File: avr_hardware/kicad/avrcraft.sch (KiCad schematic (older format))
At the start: 55 parts, among them J1 AVRISP6, P1 ETHERNET, P2 CONN_1, P3 CONN_1, P4 CONN_1, P5 CONN_1, P6 CONN_1, P7 CONN_1, P8 CONN_1, Q1 MOSFET_P, T1 S553-5999-52, U1 ATMEGA328, U2 MCP1824, U3 ENC424J600, U4 A4447SLJTR, X1 XTAL4P, X2 25MHz

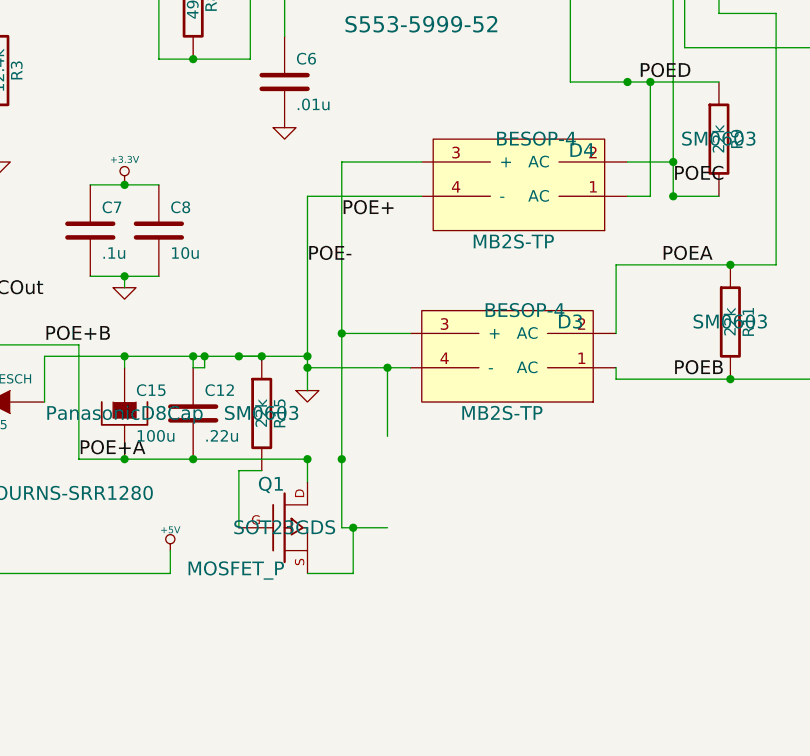
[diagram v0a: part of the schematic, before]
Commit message: update files for actual hardware
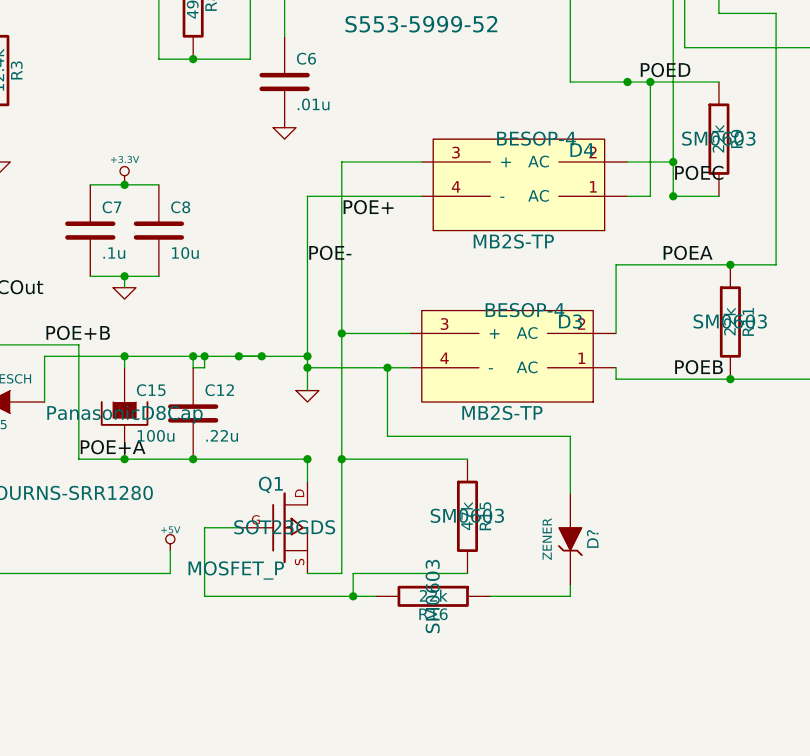
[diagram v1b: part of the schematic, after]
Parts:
- added D?: ZENER, symbol ZENER
- added R16: 22k, SM0603, symbol R
- C6: footprint SM0805 -> SM0603
- R15: value 22k -> 47k
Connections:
- net GND: now also D?.1 (A); no longer R15.1
- net POE+: now also R15.1
- net at Q1.G, R15.2: now also R16.2
- new net: D?.2 (K), R16.1
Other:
- moved on the sheet: R15
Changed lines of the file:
@@
-EESchema Schematic File Version 2  date Thu 31 Jan 2013 12:07:58 AM EST
+EESchema Schematic File Version 2  date Sun 03 Feb 2013 12:44:29 AM EST
 LIBS:power
 LIBS:device
@@
 LIBS:a4447sljtr
 LIBS:crystal-4p
+LIBS:zener-sot23-3
 LIBS:avrcraft-cache
 EELAYER 25  0
@@
 Sheet 1 1
 Title ""
-Date "31 jan 2013"
+Date "3 feb 2013"
 Rev ""
 Comp ""
@@
 Comment4 ""
 $EndDescr
-Text Label 7750 6450 0    60   ~ 0
-POE+A
+Wire Wire Line
+	9900 7000 9900 7050
+Wire Wire Line
+	8750 6950 8900 6950
+Wire Wire Line
+	8900 6950 8900 5150
+Wire Wire Line
+	9900 7050 9550 7050
 Wire Wire Line
 	8750 6450 7750 6450
@@
 Connection ~ 9100 6050
 Wire Wire Line
-	9100 6350 9100 6050
+	9100 6050 9100 6350
 Connection ~ 3800 1800
 Wire Wire Line
@@
 Connection ~ 10600 6100
 Wire Wire Line
-	9250 5150 8900 5150
+	8900 5150 9250 5150
 Wire Wire Line
 	9250 5300 8750 5300
@@
 Wire Wire Line
 	1400 2800 2000 2800
-Wire Wire Line
-	8900 5150 8900 6750
-Wire Wire Line
-	8900 6750 9100 6750
 Connection ~ 8900 6450
-Wire Wire Line
-	8750 6950 8950 6950
-Wire Wire Line
-	8950 6950 8950 6750
-Connection ~ 8950 6750
 Wire Wire Line
 	7950 6050 7950 6000
@@
 Connection ~ 8750 6450
 Wire Wire Line
-	8550 6500 8450 6500
-Wire Wire Line
-	8450 6500 8450 6750
+	8900 6450 9450 6450
+Wire Wire Line
+	9100 6350 9900 6350
+Wire Wire Line
+	9900 6350 9900 6600
+Wire Wire Line
+	9050 7050 8300 7050
+Wire Wire Line
+	8300 7050 8300 6750
+Wire Wire Line
+	8300 6750 8450 6750
+Wire Wire Line
+	9450 6950 8950 6950
+Wire Wire Line
+	8950 6950 8950 7050
+Connection ~ 8950 7050
+$Comp
+L ZENER D?
+U 1 1 510DF933
+P 9900 6800
+F 0 "D?" H 9900 6900 50  0000 C CNN
+F 1 "ZENER" H 9900 6700 40  0000 C CNN
+	1    9900 6800
+	0    1    1    0
+$EndComp
+$Comp
+L R R16
+U 1 1 510DEE44
+P 9300 7050
+F 0 "R16" V 9380 7050 50  0000 C CNN
+F 1 "22k" V 9300 7050 50  0000 C CNN
+F 2 "SM0603" H 9300 7050 60  0000 C CNN
+	1    9300 7050
+	0    1    1    0
+$EndComp
+Text Label 7750 6450 0    60   ~ 0
+POE+A
 $Comp
 L R R15
 U 1 1 5109F770
-P 8550 6250
-F 0 "R15" V 8630 6250 50  0000 C CNN
-F 1 "22k" V 8550 6250 50  0000 C CNN
-F 2 "SM0603" H 8550 6250 60  0000 C CNN
-	1    8550 6250
+P 9450 6700
+F 0 "R15" V 9530 6700 50  0000 C CNN
+F 1 "47k" V 9450 6700 50  0000 C CNN
+F 2 "SM0603" H 9450 6700 60  0000 C CNN
+	1    9450 6700
 	1    0    0    -1
 $EndComp
@@
 F 0 "C6" H 8700 4900 50  0000 L CNN
 F 1 ".01u" H 8700 4700 50  0000 L CNN
-F 2 "SM0805" H 8650 4800 60  0001 C CNN
+F 2 "SM0603" H 8650 4800 60  0001 C CNN
 	1    8650 4800
 	1    0    0    -1
